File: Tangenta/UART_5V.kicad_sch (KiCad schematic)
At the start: 13 parts, among them J15 Conn_01x06_Pin, Q3 BSS138

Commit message: Libraries exported from global to project.
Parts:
- J15: symbol Connector:Conn_01x06_Pin -> CholaSymbolsPrjLib:Conn_01x06_Pin
- Q3: symbol Transistor_FET:BSS138 -> CholaSymbolsPrjLib:BSS138
- R2: symbol Device:R_Small_US -> CholaSymbolsPrjLib:R_Small_US
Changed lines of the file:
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@@
     (effects (font (size 1.27 1.27)) (justify right))
   )
-  (symbol (lib_id "Device:R_Small_US") (at 133.985 58.42 180) (unit 1)
+  (symbol (lib_id "CholaSymbolsPrjLib:R_Small_US") (at 133.985 58.42 180) (unit 1)
     (in_bom yes) (on_board yes) (dnp no)
     (property "Reference" "R2" (at 132.715 57.15 0)
@@
     )
   )
-  (symbol (lib_id "Device:R_Small_US") (at 160.655 100.33 180) (unit 1)
+  (symbol (lib_id "CholaSymbolsPrjLib:R_Small_US") (at 160.655 100.33 180) (unit 1)
     (in_bom yes) (on_board yes) (dnp no)
     (property "Reference" "R2" (at 159.385 99.06 0)
@@
     )
   )
-  (symbol (lib_id "Connector:Conn_01x06_Pin") (at 230.505 90.805 0) (mirror y) (unit 1)
+  (symbol (lib_id "CholaSymbolsPrjLib:Conn_01x06_Pin") (at 230.505 90.805 0) (mirror y) (unit 1)
     (in_bom yes) (on_board yes) (dnp no)
     (property "Reference" "J15" (at 233.426 91.948 0)
@@
     )
   )
-  (symbol (lib_id "Transistor_FET:BSS138") (at 146.685 83.185 270) (unit 1)
+  (symbol (lib_id "CholaSymbolsPrjLib:BSS138") (at 146.685 83.185 270) (unit 1)
     (in_bom yes) (on_board yes) (dnp no)
     (property "Reference" "Q3" (at 149.225 80.645 90)
@@
     )
   )
-  (symbol (lib_id "Transistor_FET:BSS138") (at 146.685 104.14 270) (unit 1)
+  (symbol (lib_id "CholaSymbolsPrjLib:BSS138") (at 146.685 104.14 270) (unit 1)
     (in_bom yes) (on_board yes) (dnp no)
     (property "Reference" "Q3" (at 149.225 101.6 90)
@@
     )
   )
-  (symbol (lib_id "Device:R_Small_US") (at 160.655 121.285 180) (unit 1)
+  (symbol (lib_id "CholaSymbolsPrjLib:R_Small_US") (at 160.655 121.285 180) (unit 1)
     (in_bom yes) (on_board yes) (dnp no)
     (property "Reference" "R2" (at 159.385 120.015 0)
@@
     )
   )
-  (symbol (lib_id "Device:R_Small_US") (at 133.985 79.375 180) (unit 1)
+  (symbol (lib_id "CholaSymbolsPrjLib:R_Small_US") (at 133.985 79.375 180) (unit 1)
     (in_bom yes) (on_board yes) (dnp no)
     (property "Reference" "R2" (at 132.715 78.105 0)
@@
     )
   )
-  (symbol (lib_id "Device:R_Small_US") (at 160.655 79.375 180) (unit 1)
+  (symbol (lib_id "CholaSymbolsPrjLib:R_Small_US") (at 160.655 79.375 180) (unit 1)
     (in_bom yes) (on_board yes) (dnp no)
     (property "Reference" "R2" (at 159.385 78.105 0)
@@
     )
   )
-  (symbol (lib_id "Transistor_FET:BSS138") (at 146.685 62.23 270) (unit 1)
+  (symbol (lib_id "CholaSymbolsPrjLib:BSS138") (at 146.685 62.23 270) (unit 1)
     (in_bom yes) (on_board yes) (dnp no)
     (property "Reference" "Q3" (at 149.225 59.69 90)
@@
     )
   )
-  (symbol (lib_id "Device:R_Small_US") (at 133.985 100.33 180) (unit 1)
+  (symbol (lib_id "CholaSymbolsPrjLib:R_Small_US") (at 133.985 100.33 180) (unit 1)
     (in_bom yes) (on_board yes) (dnp no)
     (property "Reference" "R2" (at 132.715 99.06 0)
@@
     )
   )
-  (symbol (lib_id "Transistor_FET:BSS138") (at 146.685 125.095 270) (unit 1)
+  (symbol (lib_id "CholaSymbolsPrjLib:BSS138") (at 146.685 125.095 270) (unit 1)
     (in_bom yes) (on_board yes) (dnp no)
     (property "Reference" "Q3" (at 149.225 122.555 90)
@@
     )
   )
-  (symbol (lib_id "Device:R_Small_US") (at 133.985 121.285 180) (unit 1)
+  (symbol (lib_id "CholaSymbolsPrjLib:R_Small_US") (at 133.985 121.285 180) (unit 1)
     (in_bom yes) (on_board yes) (dnp no)
     (property "Reference" "R2" (at 132.715 120.015 0)
@@
     )
   )
-  (symbol (lib_id "Device:R_Small_US") (at 160.655 58.42 180) (unit 1)
+  (symbol (lib_id "CholaSymbolsPrjLib:R_Small_US") (at 160.655 58.42 180) (unit 1)
     (in_bom yes) (on_board yes) (dnp no)
     (property "Reference" "R2" (at 159.385 57.15 0)

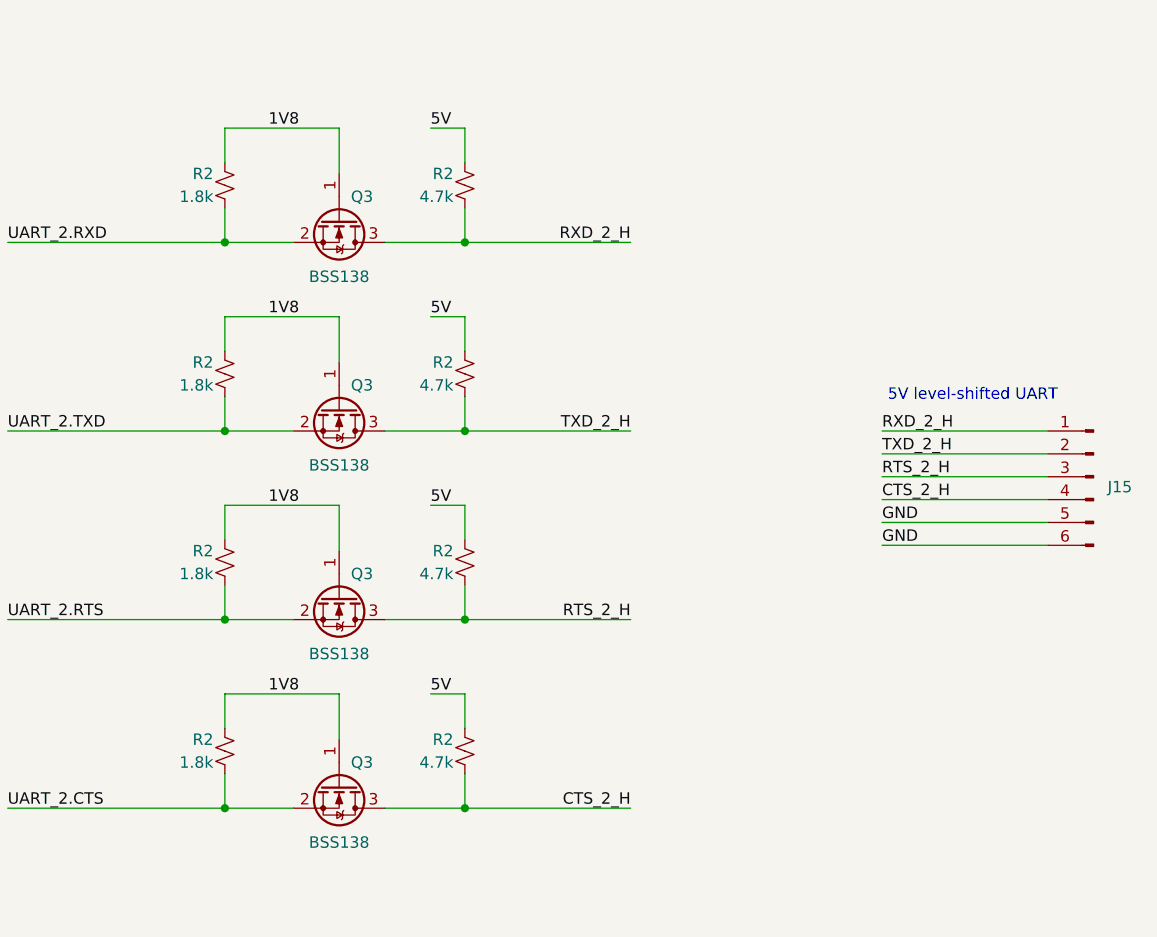
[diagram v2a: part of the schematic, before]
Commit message: initialize branch
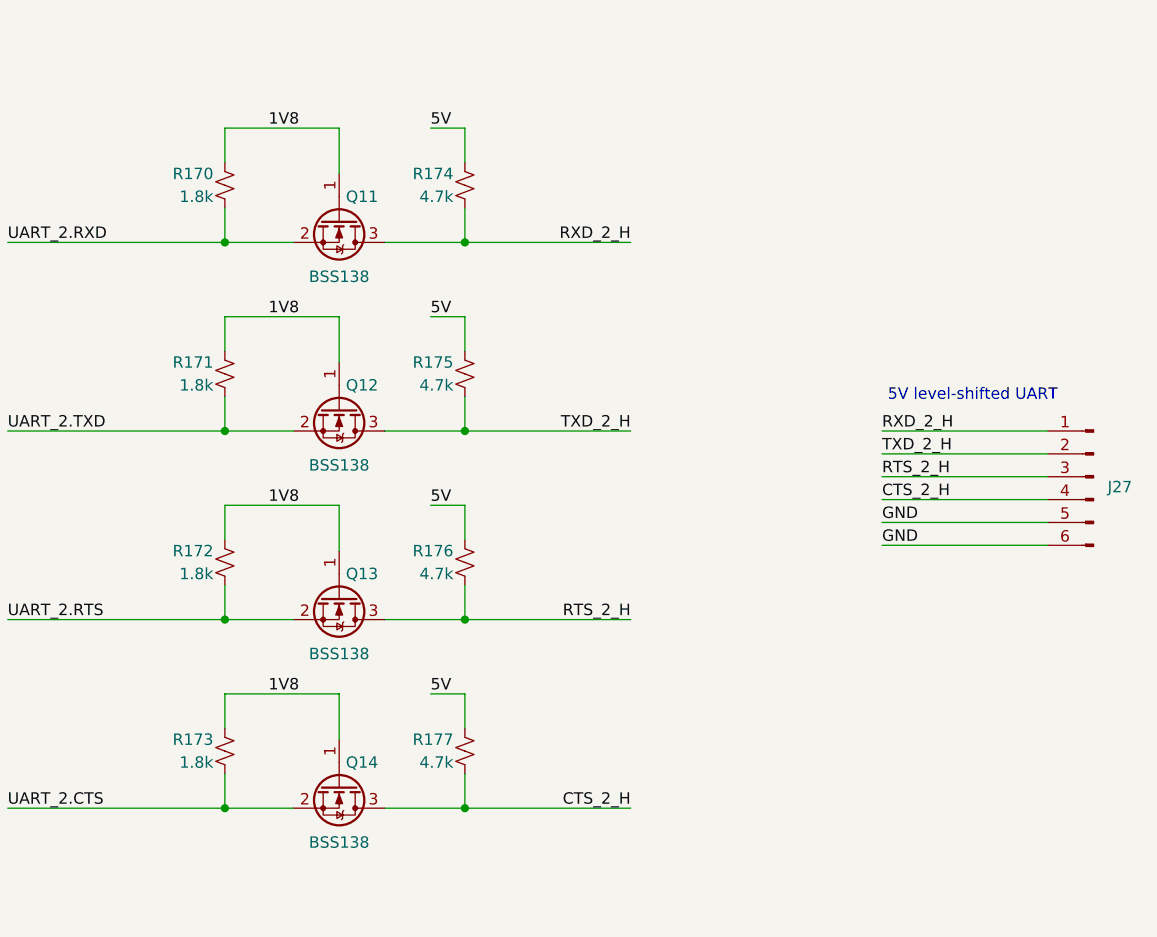
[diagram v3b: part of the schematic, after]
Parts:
- renumbered J15 to J27, Q3 to Q11, Q3 to Q12, Q3 to Q13, Q3 to Q14, R2 to R170, R2 to R171, R2 to R172, R2 to R173, R2 to R174, R2 to R175, R2 to R176, R2 to R177

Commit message: Removing component association with previous project (local) libraries.
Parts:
- J27: symbol CholaSymbolsPrjLib:Conn_01x06_Pin -> Conn_01x06_Pin:Conn_01x06_Pin
- Q11, Q12, Q13, Q14: symbol CholaSymbolsPrjLib:BSS138 -> BSS138:BSS138
- R170, R171, R172, R173, R174, R175, R176, R177: symbol CholaSymbolsPrjLib:R_Small_US -> R_Small_US:R_Small_US
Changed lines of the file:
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@@
 	)
 	(symbol
-		(lib_id "CholaSymbolsPrjLib:R_Small_US")
+		(lib_id "R_Small_US:R_Small_US")
 		(at 133.985 58.42 180)
 		(unit 1)
@@
 	)
 	(symbol
-		(lib_id "CholaSymbolsPrjLib:R_Small_US")
+		(lib_id "R_Small_US:R_Small_US")
 		(at 160.655 100.33 180)
 		(unit 1)
@@
 	)
 	(symbol
-		(lib_id "CholaSymbolsPrjLib:Conn_01x06_Pin")
+		(lib_id "Conn_01x06_Pin:Conn_01x06_Pin")
 		(at 230.505 90.805 0)
 		(mirror y)
@@
 	)
 	(symbol
-		(lib_id "CholaSymbolsPrjLib:BSS138")
+		(lib_id "BSS138:BSS138")
 		(at 146.685 83.185 270)
 		(unit 1)
@@
 	)
 	(symbol
-		(lib_id "CholaSymbolsPrjLib:BSS138")
+		(lib_id "BSS138:BSS138")
 		(at 146.685 104.14 270)
 		(unit 1)
@@
 	)
 	(symbol
-		(lib_id "CholaSymbolsPrjLib:R_Small_US")
+		(lib_id "R_Small_US:R_Small_US")
 		(at 160.655 121.285 180)
 		(unit 1)
@@
 	)
 	(symbol
-		(lib_id "CholaSymbolsPrjLib:R_Small_US")
+		(lib_id "R_Small_US:R_Small_US")
 		(at 133.985 79.375 180)
 		(unit 1)
@@
 	)
 	(symbol
-		(lib_id "CholaSymbolsPrjLib:R_Small_US")
+		(lib_id "R_Small_US:R_Small_US")
 		(at 160.655 79.375 180)
 		(unit 1)
@@
 	)
 	(symbol
-		(lib_id "CholaSymbolsPrjLib:BSS138")
+		(lib_id "BSS138:BSS138")
 		(at 146.685 62.23 270)
 		(unit 1)
@@
 	)
 	(symbol
-		(lib_id "CholaSymbolsPrjLib:R_Small_US")
+		(lib_id "R_Small_US:R_Small_US")
 		(at 133.985 100.33 180)
 		(unit 1)
@@
 	)
 	(symbol
-		(lib_id "CholaSymbolsPrjLib:BSS138")
+		(lib_id "BSS138:BSS138")
 		(at 146.685 125.095 270)
 		(unit 1)
@@
 	)
 	(symbol
-		(lib_id "CholaSymbolsPrjLib:R_Small_US")
+		(lib_id "R_Small_US:R_Small_US")
 		(at 133.985 121.285 180)
 		(unit 1)
@@
 	)
 	(symbol
-		(lib_id "CholaSymbolsPrjLib:R_Small_US")
+		(lib_id "R_Small_US:R_Small_US")
 		(at 160.655 58.42 180)
 		(unit 1)

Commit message: Fixes, continued...
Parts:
- J27: symbol Conn_01x06_Pin:Conn_01x06_Pin -> Connector_Generic:Conn_01x06_Pin
- Q11, Q12, Q13, Q14: symbol BSS138:BSS138 -> Transistor_FET:BSS138
- R170, R171, R172, R173, R174, R175, R176, R177: symbol R_Small_US:R_Small_US -> Device:R_Small_US
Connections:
- net 1V8: no longer Q11.1 (G), Q12.1 (G), Q13.1 (G), Q14.1 (G), R170.2, R171.2, R172.2, R173.2
- net 5V: no longer R174.2, R175.2, R176.2, R177.2
- net CTS_2_H: no longer J27.4 (Pin_4), Q14.3 (D), R177.1
- net GNDREF: no longer J27.5 (Pin_5), J27.6 (Pin_6)
- net RTS_2_H: no longer J27.3 (Pin_3), Q13.3 (D), R176.1
- net RXD_2_H: no longer J27.1 (Pin_1), Q11.3 (D), R174.1
- net TXD_2_H: no longer J27.2 (Pin_2), Q12.3 (D), R175.1
- net UART_2.CTS: no longer Q14.2 (S), R173.1
- net UART_2.RTS: no longer Q13.2 (S), R172.1
- net UART_2.RXD: no longer Q11.2 (S), R170.1
- net UART_2.TXD: no longer Q12.2 (S), R171.1
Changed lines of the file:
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@@
 	)
 	(symbol
-		(lib_id "R_Small_US:R_Small_US")
+		(lib_id "Device:R_Small_US")
 		(at 133.985 58.42 180)
 		(unit 1)
@@
 	)
 	(symbol
-		(lib_id "R_Small_US:R_Small_US")
+		(lib_id "Device:R_Small_US")
 		(at 160.655 100.33 180)
 		(unit 1)
@@
 	)
 	(symbol
-		(lib_id "Conn_01x06_Pin:Conn_01x06_Pin")
+		(lib_id "Connector_Generic:Conn_01x06_Pin")
 		(at 230.505 90.805 0)
 		(mirror y)
@@
 	)
 	(symbol
-		(lib_id "BSS138:BSS138")
+		(lib_id "Transistor_FET:BSS138")
 		(at 146.685 83.185 270)
 		(unit 1)
@@
 	)
 	(symbol
-		(lib_id "BSS138:BSS138")
+		(lib_id "Transistor_FET:BSS138")
 		(at 146.685 104.14 270)
 		(unit 1)
@@
 	)
 	(symbol
-		(lib_id "R_Small_US:R_Small_US")
+		(lib_id "Device:R_Small_US")
 		(at 160.655 121.285 180)
 		(unit 1)
@@
 	)
 	(symbol
-		(lib_id "R_Small_US:R_Small_US")
+		(lib_id "Device:R_Small_US")
 		(at 133.985 79.375 180)
 		(unit 1)
@@
 	)
 	(symbol
-		(lib_id "R_Small_US:R_Small_US")
+		(lib_id "Device:R_Small_US")
 		(at 160.655 79.375 180)
 		(unit 1)
@@
 	)
 	(symbol
-		(lib_id "BSS138:BSS138")
+		(lib_id "Transistor_FET:BSS138")
 		(at 146.685 62.23 270)
 		(unit 1)
@@
 	)
 	(symbol
-		(lib_id "R_Small_US:R_Small_US")
+		(lib_id "Device:R_Small_US")
 		(at 133.985 100.33 180)
 		(unit 1)
@@
 	)
 	(symbol
-		(lib_id "BSS138:BSS138")
+		(lib_id "Transistor_FET:BSS138")
 		(at 146.685 125.095 270)
 		(unit 1)
@@
 	)
 	(symbol
-		(lib_id "R_Small_US:R_Small_US")
+		(lib_id "Device:R_Small_US")
 		(at 133.985 121.285 180)
 		(unit 1)
@@
 	)
 	(symbol
-		(lib_id "R_Small_US:R_Small_US")
+		(lib_id "Device:R_Small_US")
 		(at 160.655 58.42 180)
 		(unit 1)

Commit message: Fixes, continued...
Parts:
- J27: symbol Connector_Generic:Conn_01x06_Pin -> Conn_01x06_Pin:Conn_01x06_Pin
- Q11, Q12, Q13, Q14: symbol Transistor_FET:BSS138 -> BSS138:BSS138
- R170, R171, R172, R173, R174, R175, R176, R177: symbol Device:R_Small_US -> R_Small_US:R_Small_US
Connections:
- net 1V8: now also Q11.1 (G), Q12.1 (G), Q13.1 (G), Q14.1 (G), R170.2, R171.2, R172.2, R173.2
- net 5V: now also R174.2, R175.2, R176.2, R177.2
- net CTS_2_H: now also J27.4 (Pin_4), Q14.3 (D), R177.1
- net GNDREF: now also J27.5 (Pin_5), J27.6 (Pin_6)
- net RTS_2_H: now also J27.3 (Pin_3), Q13.3 (D), R176.1
- net RXD_2_H: now also J27.1 (Pin_1), Q11.3 (D), R174.1
- net TXD_2_H: now also J27.2 (Pin_2), Q12.3 (D), R175.1
- net UART_2.CTS: now also Q14.2 (S), R173.1
- net UART_2.RTS: now also Q13.2 (S), R172.1
- net UART_2.RXD: now also Q11.2 (S), R170.1
- net UART_2.TXD: now also Q12.2 (S), R171.1
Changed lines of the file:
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@@
 	)
 	(symbol
-		(lib_id "Device:R_Small_US")
+		(lib_id "R_Small_US:R_Small_US")
 		(at 133.985 58.42 180)
 		(unit 1)
@@
 	)
 	(symbol
-		(lib_id "Device:R_Small_US")
+		(lib_id "R_Small_US:R_Small_US")
 		(at 160.655 100.33 180)
 		(unit 1)
@@
 	)
 	(symbol
-		(lib_id "Connector_Generic:Conn_01x06_Pin")
+		(lib_id "Conn_01x06_Pin:Conn_01x06_Pin")
 		(at 230.505 90.805 0)
 		(mirror y)
@@
 	)
 	(symbol
-		(lib_id "Transistor_FET:BSS138")
+		(lib_id "BSS138:BSS138")
 		(at 146.685 83.185 270)
 		(unit 1)
@@
 	)
 	(symbol
-		(lib_id "Transistor_FET:BSS138")
+		(lib_id "BSS138:BSS138")
 		(at 146.685 104.14 270)
 		(unit 1)
@@
 	)
 	(symbol
-		(lib_id "Device:R_Small_US")
+		(lib_id "R_Small_US:R_Small_US")
 		(at 160.655 121.285 180)
 		(unit 1)
@@
 	)
 	(symbol
-		(lib_id "Device:R_Small_US")
+		(lib_id "R_Small_US:R_Small_US")
 		(at 133.985 79.375 180)
 		(unit 1)
@@
 	)
 	(symbol
-		(lib_id "Device:R_Small_US")
+		(lib_id "R_Small_US:R_Small_US")
 		(at 160.655 79.375 180)
 		(unit 1)
@@
 	)
 	(symbol
-		(lib_id "Transistor_FET:BSS138")
+		(lib_id "BSS138:BSS138")
 		(at 146.685 62.23 270)
 		(unit 1)
@@
 	)
 	(symbol
-		(lib_id "Device:R_Small_US")
+		(lib_id "R_Small_US:R_Small_US")
 		(at 133.985 100.33 180)
 		(unit 1)
@@
 	)
 	(symbol
-		(lib_id "Transistor_FET:BSS138")
+		(lib_id "BSS138:BSS138")
 		(at 146.685 125.095 270)
 		(unit 1)
@@
 	)
 	(symbol
-		(lib_id "Device:R_Small_US")
+		(lib_id "R_Small_US:R_Small_US")
 		(at 133.985 121.285 180)
 		(unit 1)
@@
 	)
 	(symbol
-		(lib_id "Device:R_Small_US")
+		(lib_id "R_Small_US:R_Small_US")
 		(at 160.655 58.42 180)
 		(unit 1)

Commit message: Fixes, before checks.
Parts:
- J27: symbol Conn_01x06_Pin:Conn_01x06_Pin -> Connector_Generic:Conn_01x06
- Q11, Q12, Q13, Q14: symbol BSS138:BSS138 -> Transistor_FET:BSS138
- R170, R171, R172, R173, R174, R175, R176, R177: symbol R_Small_US:R_Small_US -> Device:R_Small_US
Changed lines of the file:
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@@
 	)
 	(symbol
-		(lib_id "R_Small_US:R_Small_US")
+		(lib_id "Device:R_Small_US")
 		(at 133.985 58.42 180)
 		(unit 1)
@@
 	)
 	(symbol
-		(lib_id "R_Small_US:R_Small_US")
+		(lib_id "Device:R_Small_US")
 		(at 160.655 100.33 180)
 		(unit 1)
@@
 	)
 	(symbol
-		(lib_id "Conn_01x06_Pin:Conn_01x06_Pin")
+		(lib_id "Connector_Generic:Conn_01x06")
 		(at 230.505 90.805 0)
 		(mirror y)
@@
 	)
 	(symbol
-		(lib_id "BSS138:BSS138")
+		(lib_id "Transistor_FET:BSS138")
 		(at 146.685 83.185 270)
 		(unit 1)
@@
 	)
 	(symbol
-		(lib_id "BSS138:BSS138")
+		(lib_id "Transistor_FET:BSS138")
 		(at 146.685 104.14 270)
 		(unit 1)
@@
 	)
 	(symbol
-		(lib_id "R_Small_US:R_Small_US")
+		(lib_id "Device:R_Small_US")
 		(at 160.655 121.285 180)
 		(unit 1)
@@
 	)
 	(symbol
-		(lib_id "R_Small_US:R_Small_US")
+		(lib_id "Device:R_Small_US")
 		(at 133.985 79.375 180)
 		(unit 1)
@@
 	)
 	(symbol
-		(lib_id "R_Small_US:R_Small_US")
+		(lib_id "Device:R_Small_US")
 		(at 160.655 79.375 180)
 		(unit 1)
@@
 	)
 	(symbol
-		(lib_id "BSS138:BSS138")
+		(lib_id "Transistor_FET:BSS138")
 		(at 146.685 62.23 270)
 		(unit 1)
@@
 	)
 	(symbol
-		(lib_id "R_Small_US:R_Small_US")
+		(lib_id "Device:R_Small_US")
 		(at 133.985 100.33 180)
 		(unit 1)
@@
 	)
 	(symbol
-		(lib_id "BSS138:BSS138")
+		(lib_id "Transistor_FET:BSS138")
 		(at 146.685 125.095 270)
 		(unit 1)
@@
 	)
 	(symbol
-		(lib_id "R_Small_US:R_Small_US")
+		(lib_id "Device:R_Small_US")
 		(at 133.985 121.285 180)
 		(unit 1)
@@
 	)
 	(symbol
-		(lib_id "R_Small_US:R_Small_US")
+		(lib_id "Device:R_Small_US")
 		(at 160.655 58.42 180)
 		(unit 1)
